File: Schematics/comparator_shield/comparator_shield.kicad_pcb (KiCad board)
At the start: 4 copper layers, 68.6 x 53.3 mm, 51 parts, among them J1 Conn_1x1_Female, J2 Conn_1x1_Female, J3 Conn_1x1_Female, J4 Conn_1x1_Female, J5 Conn_1x1_Female, J6 Conn_1x1_Female, J7 Conn_1x1_Female, J8 Conn_1x1_Female, J9 Conn_1x1_Female, U1 TLV3704

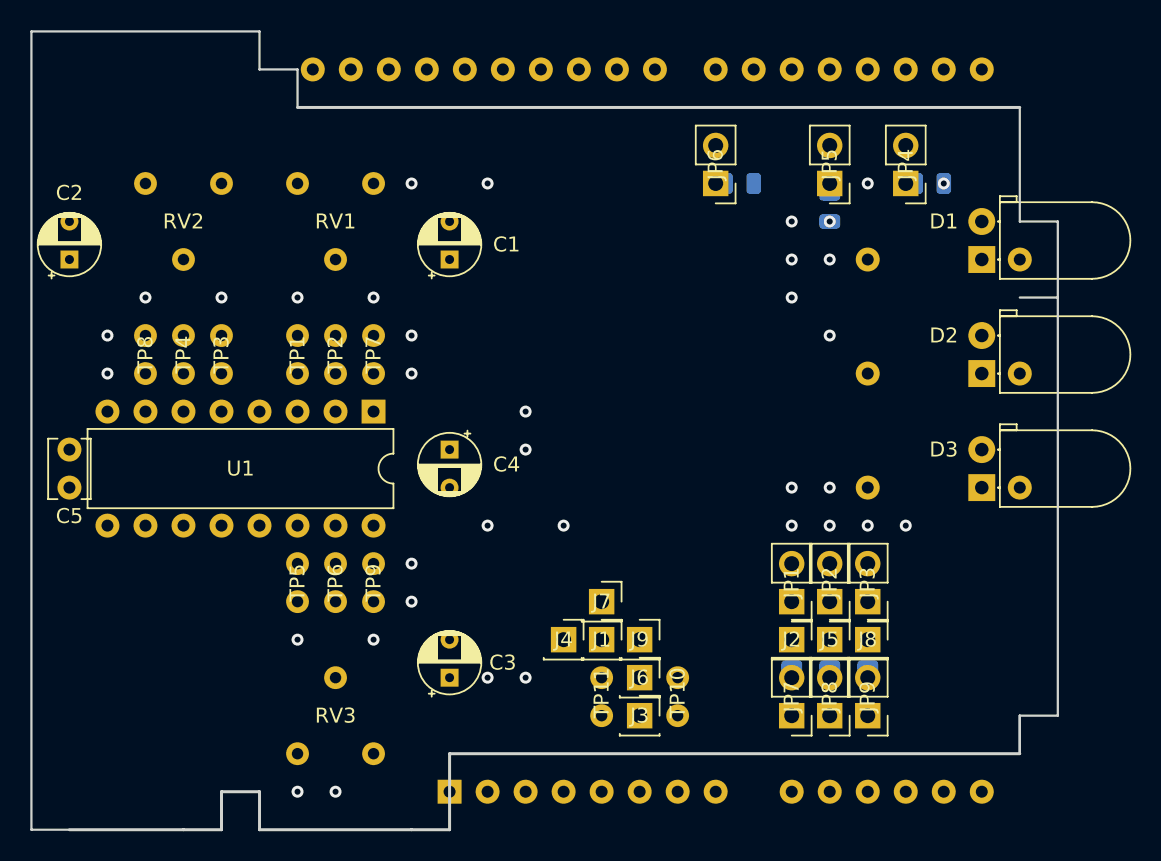
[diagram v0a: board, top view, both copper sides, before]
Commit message: added some changes
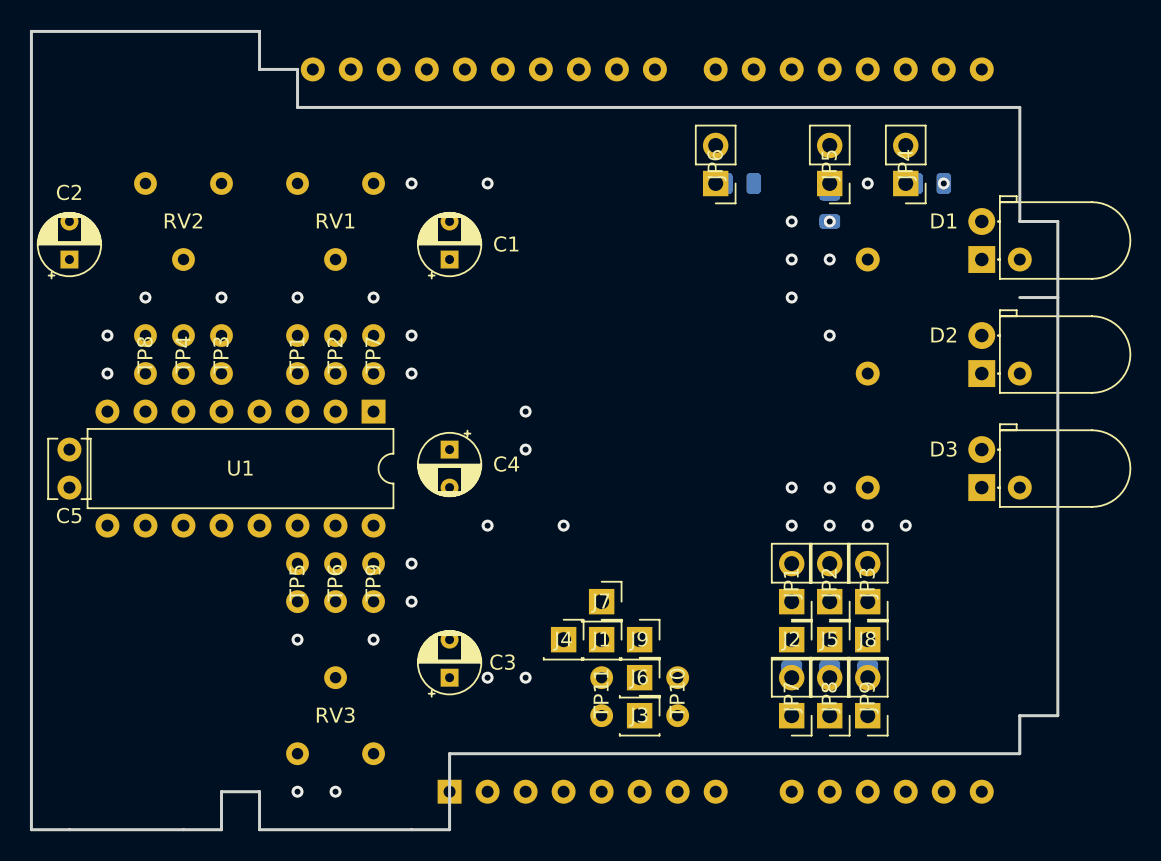
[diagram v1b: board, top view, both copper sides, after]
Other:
- board text removed: "misc_shield.kicad_pcb"
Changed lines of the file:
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@@
   (general
     (thickness 1.6)
-    (drawings 29)
+    (drawings 28)
     (tracks 227)
     (zones 0)
@@
     )
   )
-  (gr_text misc_shield.kicad_pcb (at 194.31 186.055) (layer Dwgs.User)
-    (effects (font (size 1.27 1.27) (thickness 0.127)))
-  )
   (gr_text - (at 269.875 193.04) (layer Dwgs.User)
     (effects (font (size 1.27 1.27) (thickness 0.127)))
@@
   (gr_line (start 139.7 132.08) (end 139.7 127) (layer Edge.Cuts) (width 0.2))
   (gr_line (start 129.54 83.82) (end 177.8 83.82) (layer Edge.Cuts) (width 0.2))
-  (gr_line (start 111.76 132.08) (end 114.3 132.08) (layer Edge.Cuts) (width 0.15))
-  (gr_line (start 111.76 78.74) (end 111.76 132.08) (layer Edge.Cuts) (width 0.15))
-  (gr_line (start 127 78.74) (end 111.76 78.74) (layer Edge.Cuts) (width 0.15))
-  (gr_line (start 127 81.28) (end 127 78.74) (layer Edge.Cuts) (width 0.15))
-  (gr_line (start 129.54 81.28) (end 127 81.28) (layer Edge.Cuts) (width 0.15))
-  (gr_line (start 129.54 83.82) (end 129.54 81.28) (layer Edge.Cuts) (width 0.15))
-  (gr_line (start 177.8 91.44) (end 177.8 83.82) (layer Edge.Cuts) (width 0.15))
-  (gr_line (start 180.34 91.44) (end 177.8 91.44) (layer Edge.Cuts) (width 0.15))
-  (gr_line (start 180.34 96.52) (end 180.34 91.44) (layer Edge.Cuts) (width 0.15))
-  (gr_line (start 180.34 96.52) (end 177.8 96.52) (layer Edge.Cuts) (width 0.15))
-  (gr_line (start 180.34 124.46) (end 180.34 96.52) (layer Edge.Cuts) (width 0.15))
-  (gr_line (start 177.8 124.46) (end 180.34 124.46) (layer Edge.Cuts) (width 0.15))
-  (gr_line (start 177.8 124.46) (end 177.8 127) (layer Edge.Cuts) (width 0.15))
+  (gr_line (start 111.76 132.08) (end 114.3 132.08) (layer Edge.Cuts) (width 0.2))
+  (gr_line (start 111.76 78.74) (end 111.76 132.08) (layer Edge.Cuts) (width 0.2))
+  (gr_line (start 127 78.74) (end 111.76 78.74) (layer Edge.Cuts) (width 0.2))
+  (gr_line (start 127 81.28) (end 127 78.74) (layer Edge.Cuts) (width 0.2))
+  (gr_line (start 129.54 81.28) (end 127 81.28) (layer Edge.Cuts) (width 0.2))
+  (gr_line (start 129.54 83.82) (end 129.54 81.28) (layer Edge.Cuts) (width 0.2))
+  (gr_line (start 177.8 91.44) (end 177.8 83.82) (layer Edge.Cuts) (width 0.2))
+  (gr_line (start 180.34 91.44) (end 177.8 91.44) (layer Edge.Cuts) (width 0.2))
+  (gr_line (start 180.34 96.52) (end 180.34 91.44) (layer Edge.Cuts) (width 0.2))
+  (gr_line (start 180.34 96.52) (end 177.8 96.52) (layer Edge.Cuts) (width 0.2))
+  (gr_line (start 180.34 124.46) (end 180.34 96.52) (layer Edge.Cuts) (width 0.2))
+  (gr_line (start 177.8 124.46) (end 180.34 124.46) (layer Edge.Cuts) (width 0.2))
+  (gr_line (start 177.8 124.46) (end 177.8 127) (layer Edge.Cuts) (width 0.2))
   (gr_line (start 177.8 127) (end 177.8 124.46) (layer Edge.Cuts) (width 0.15))
   (gr_line (start 137.16 132.08) (end 139.7 132.08) (layer Edge.Cuts) (width 0.2))
